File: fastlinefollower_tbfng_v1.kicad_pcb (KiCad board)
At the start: 2 copper layers, 100 x 70 mm, 10 parts, among them J1 IR_conn, J2 Motor1, J3 Motor2, SW1 Run, SW2 Calibrate, U1 TB6612FNG_Module, U2 LM7805_TO220

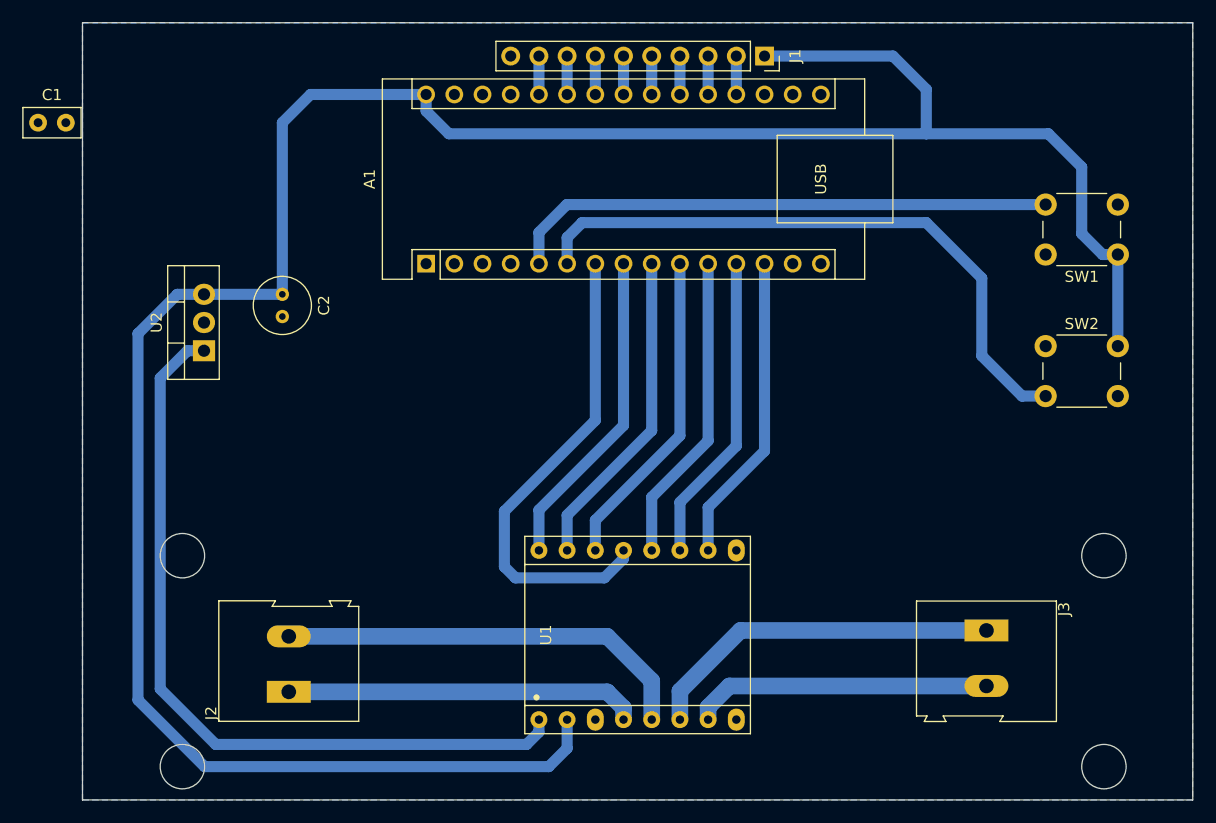
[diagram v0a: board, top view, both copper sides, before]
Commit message: well theres a second version now
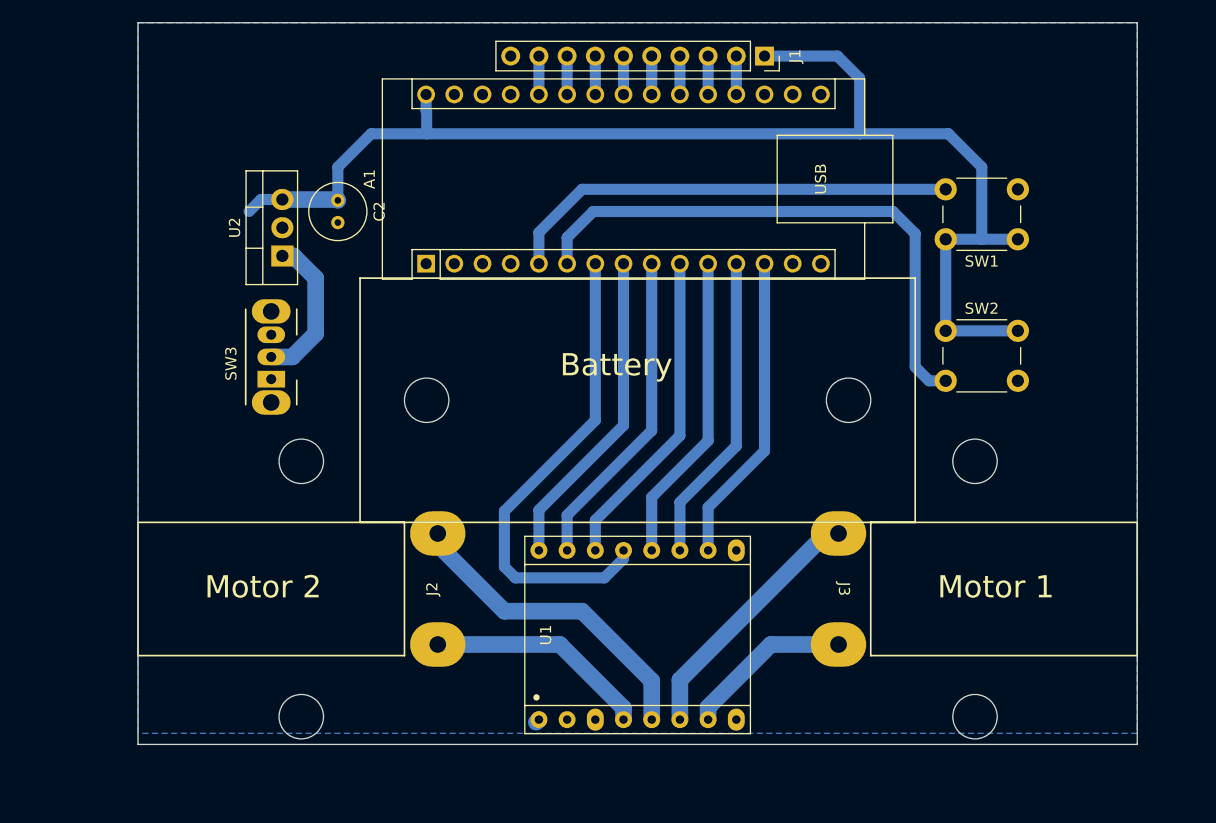
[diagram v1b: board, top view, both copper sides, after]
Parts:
- removed C1: C, Capacitor_THT:C_Disc_D5.0mm_W2.5mm_P2.50mm
- added SW3: SW_SPST, Button_Switch_THT:SW_CuK_OS102011MA1QN1_SPDT_Angled, F.Cu at (108.0, 123.1)
- J2, J3: footprint TerminalBlock:TerminalBlock_Altech_AK300-2_P5.00mm -> sche:MOTORmount
- moved J2 16.3 mm to (123.0, 142.0)
- moved J3 13.8 mm to (159.1, 142.0)
- moved U2 11.1 mm to (109.0, 112.0)
- moved C2 9.83 mm to (114.0, 107.0)
- moved SW1 9.10 mm to (175.2, 110.5)
- moved SW2 9.10 mm to (168.8, 118.8)
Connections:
- U2 pad 1: VS -> Net-(SW3-B)
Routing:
- net +5V: track 222.1 -> 117.7 mm
- net VS: track 70.7 -> 0.33 mm
- net Net-(SW3-B): track 0.00 -> 13.7 mm
- net /M2_B: track 27.0 -> 15.2 mm
- net /M1_A: track 31.8 -> 20.1 mm
- net /M2_A: track 32.4 -> 23.3 mm
- net /M1_B: track 37.8 -> 28.8 mm
- net /RUN: track 49.5 -> 41.1 mm
- net /CAL: track 56.6 -> 50.8 mm
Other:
- board size 100 x 70 mm -> 90 x 65 mm
- board text added: "Battery"
- board text added: "Motor 1"
- board text added: "Motor 2"
